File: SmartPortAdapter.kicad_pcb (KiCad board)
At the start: 2 copper layers, 26.4 x 34.6 mm, 11 parts, among them J1 APPLE_SDISKII, J2 Data Pin, J3 PHx/SEL

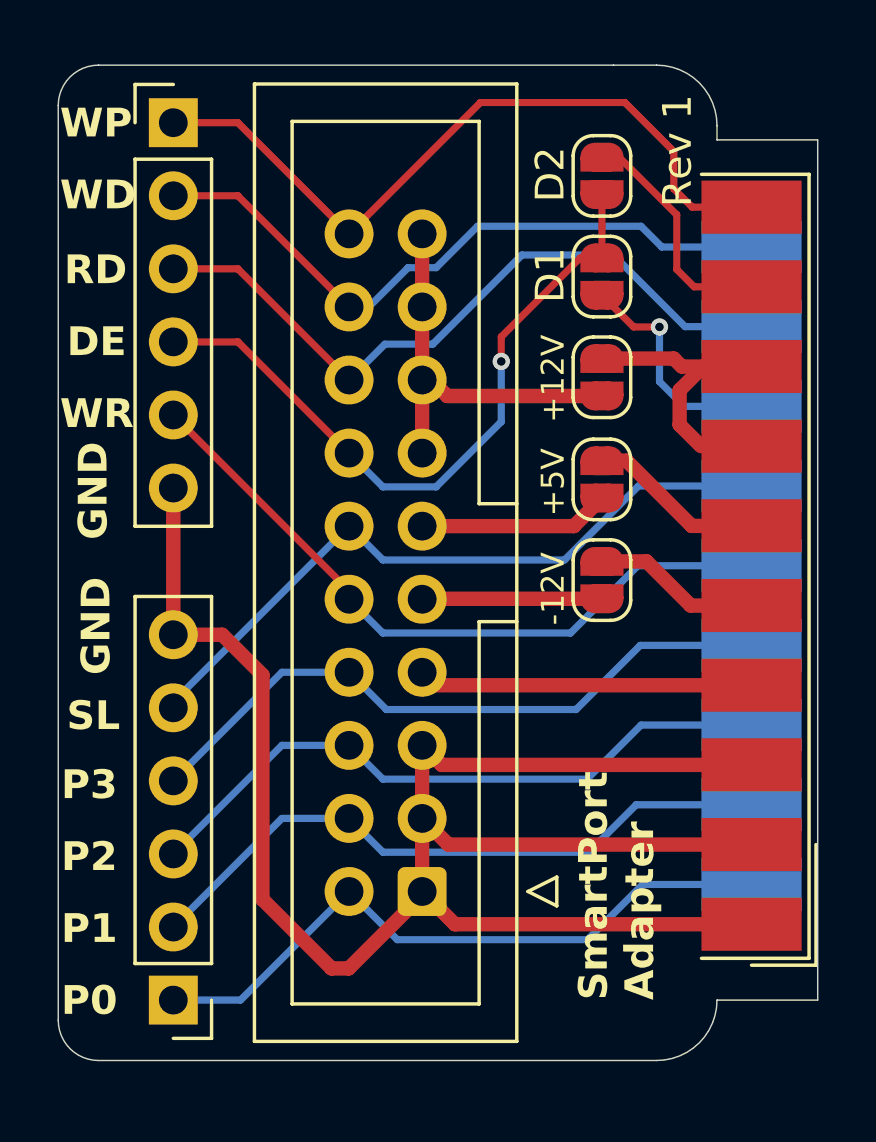
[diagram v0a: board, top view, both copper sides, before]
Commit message: rev3 IIGS ROM3
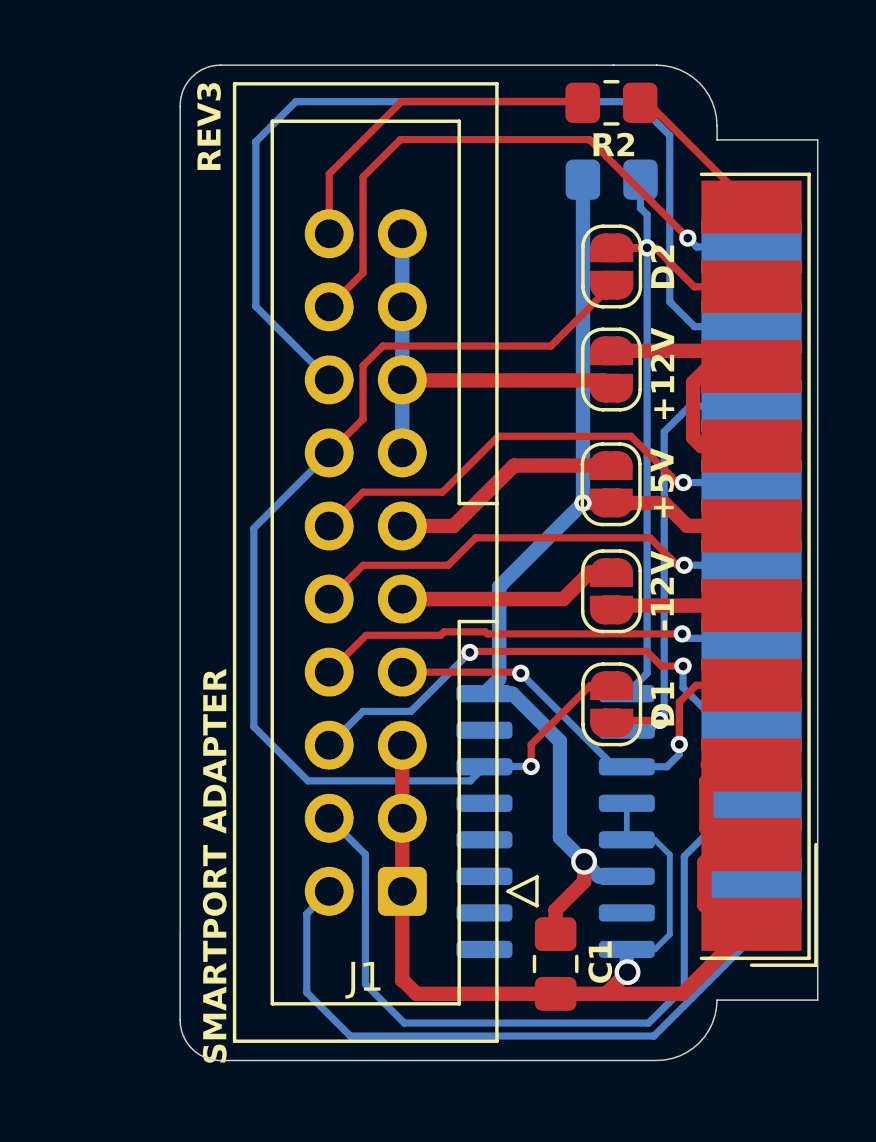
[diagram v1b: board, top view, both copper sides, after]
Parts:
- removed the   at (160.2, 108.8)
- removed the   at (161.2, 87.9)
- removed J2: Data Pin, Connector_PinHeader_2.54mm:PinHeader_1x06_P2.54mm_Vertical
- removed J3: PHx/SEL, Connector_PinHeader_2.54mm:PinHeader_1x06_P2.54mm_Vertical
- added  : LOGO, LOGO, B.Cu at (154.0, 81.5)
- added C1: 100nf, Capacitor_SMD:C_0805_2012Metric_Pad1.18x1.45mm_HandSolder, F.Cu at (159.9, 110.7)
- added G***: LOGO, Stm32F411:snap, B.Cu at (160.7, 92.6)
- added R1: 10K, Resistor_SMD:R_0805_2012Metric_Pad1.20x1.40mm_HandSolder, B.Cu at (161.8, 83.5)
- added R2: 470, Resistor_SMD:R_0805_2012Metric_Pad1.20x1.40mm_HandSolder, F.Cu at (161.8, 80.8)
- added U2: 74HC138, Package_SO:SOIC-16_3.9x9.9mm_P1.27mm, B.Cu at (159.9, 105.8)
- moved D1 14.9 mm to (161.8, 101.7)
- moved D2 3.17 mm to (161.8, 86.5)
- moved J1 0.69 mm to (154.6, 108.2)
- moved -12V 0.51 mm to (161.8, 97.8), turned to -90 degrees
- moved +12V 0.43 mm to (161.8, 90.1)
- moved +5V 0.36 mm to (161.8, 94.1), turned to -90 degrees
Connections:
- net GND4 renamed EN35
- J1 pad 20: WR_PROTECT -> WR_PROTECT_D
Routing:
- net VCC: track 6.14 -> 38.6 mm, vias 0 -> 2
- net GND: track 65.3 -> 44.4 mm, vias 0 -> 1
- net WR_PROTECT: track 26.2 -> 5.65 mm
- net DEVICE_ENABLE2: track 8.18 -> 24.9 mm, vias 0 -> 1
- net DEVICE_ENABLE_D: track 24.2 -> 39.0 mm
- net WR_PROTECT_D: track 0.00 -> 12.0 mm
- net RD_DATA: track 24.5 -> 33.8 mm
- net WR_REQ: track 24.4 -> 16.0 mm, vias 0 -> 1
- net DEVICE_ENABLE: track 8.55 -> 16.5 mm
- net SEL: track 24.4 -> 16.7 mm, vias 0 -> 1
- net STEP3: track 23.1 -> 15.5 mm, vias 0 -> 1
- net STEP2: track 22.9 -> 17.5 mm, vias 0 -> 2
- net STEP1: track 22.8 -> 27.4 mm
- net EN35: track 11.6 -> 15.7 mm, vias 0 -> 2
- net WR_DATA: track 23.2 -> 20.6 mm, vias 0 -> 1
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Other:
- board size 26.4 x 34.6 mm -> 22.2 x 34.6 mm
- board text added: "74LS138"
- board text added: "REV3"
- board text added: "SMARTPORT ADAPTER"
- board text removed: "DE"
- board text removed: "GND"
- board text removed: "P0"
- board text removed: "P1"
- board text removed: "P2"
- board text removed: "P3"
- board text removed: "RD"
- board text removed: "Rev 1"
- board text removed: "SL"
- board text removed: "SmartPort Adapter"
- board text removed: "WD"
- board text removed: "WP"
- board text removed: "WR"
